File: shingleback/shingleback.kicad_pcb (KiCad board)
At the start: 2 copper layers, 117.8 x 86.2 mm, 45 parts

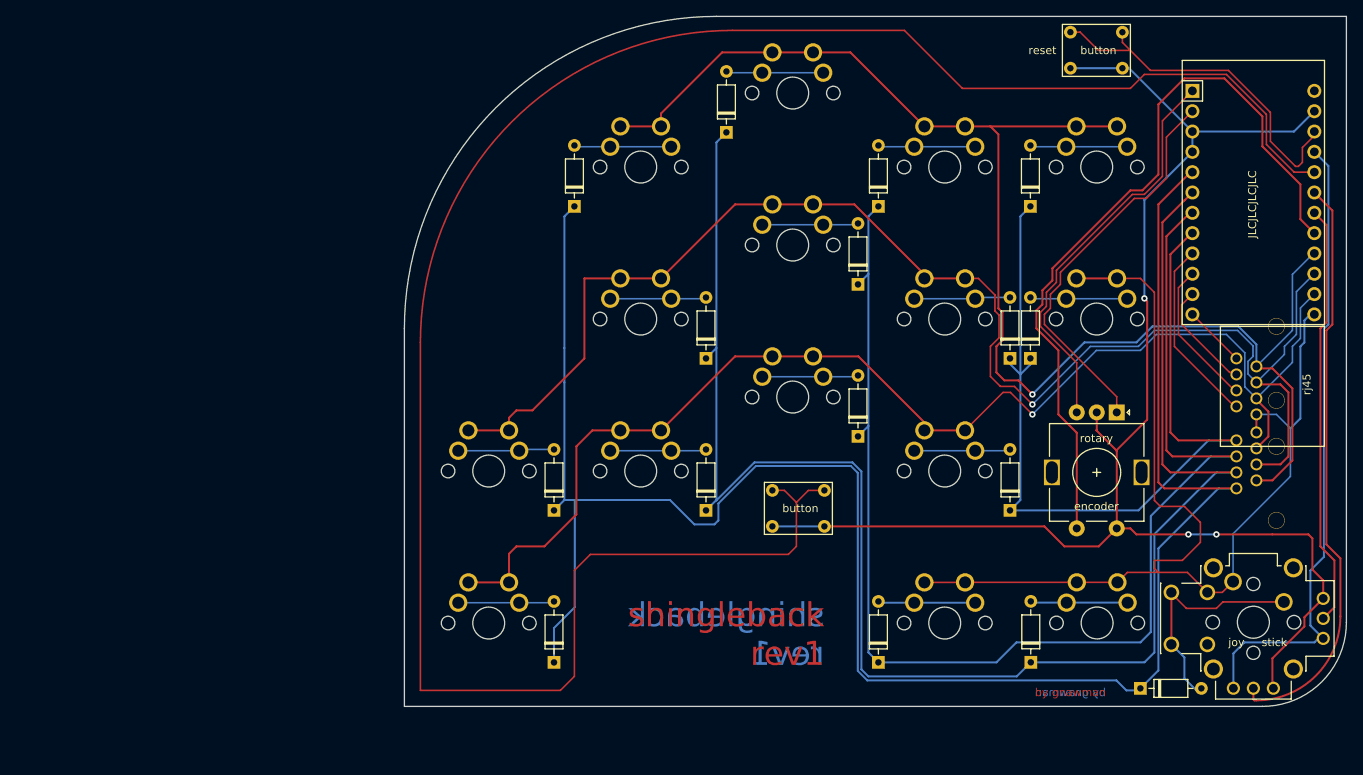
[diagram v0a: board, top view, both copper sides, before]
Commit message: shingleback rev2
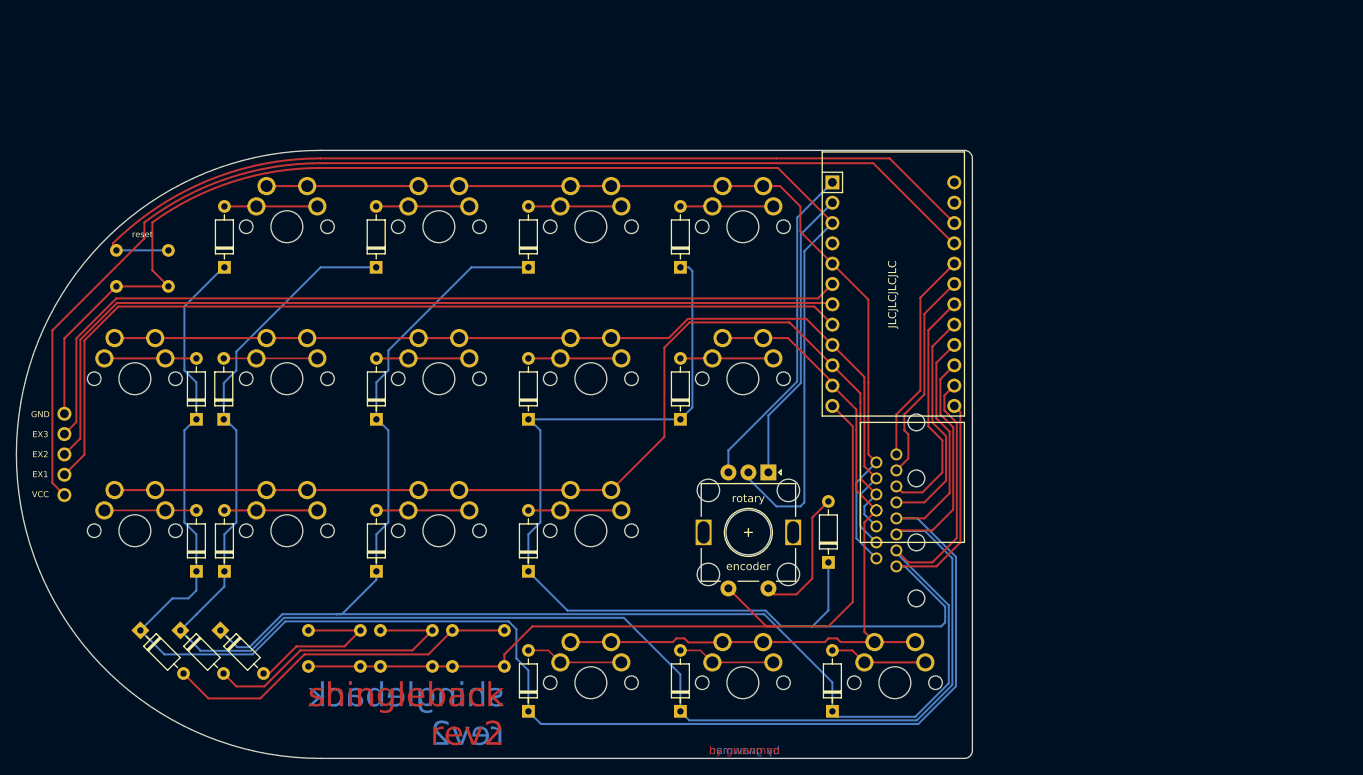
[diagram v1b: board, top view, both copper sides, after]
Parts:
- removed the ? at (125.0, 83.5)
- removed the ? at (162.2, 30.7)
- removed the ? at (118.5, 88.0)
- removed the ? at (125.0, 88.0)
- removed the ? at (155.8, 30.7)
- removed the ? at (118.5, 83.5)
- removed the ? at (155.8, 26.2)
- removed the ? at (162.2, 26.2)
- removed the R at (131.8, 105.0)
- removed the R at (150.8, 67.0)
- removed the R at (93.8, 48.0)
- removed the R at (164.5, 108.2)
- removed the R at (150.8, 105.0)
- removed the R at (129.2, 57.8)
- removed the R at (131.8, 48.0)
- removed the R at (148.2, 67.0)
- removed the R at (150.8, 48.0)
- removed the R at (110.2, 67.0)
- removed the R at (129.2, 76.8)
- removed the R at (91.2, 86.0)
- removed the R at (91.2, 105.0)
- removed the R at (112.8, 38.8)
- removed the R at (110.2, 86.0)
- removed the R at (148.2, 86.0)
- removed the REF at (185.0, 62.0)
- removed the REF at (185.0, 88.2)
- removed the REF** at (161.5, 73.8)
- removed the REF** at (183.7, 100.8)
- removed the REF** at (176.1, 94.9)
- removed the S14 at (159.0, 62.1)
- removed the S14 at (140.0, 62.1)
- removed the S14 at (121.0, 71.8)
- removed the S14 at (140.0, 81.1)
- removed the S14 at (102.0, 81.1)
- removed the S14 at (121.0, 52.8)
- removed the S14 at (140.0, 100.1)
- removed the S14 at (121.0, 33.8)
- removed the S14 at (102.0, 43.1)
- removed the S14 at (140.0, 43.1)
- removed the S14 at (159.1, 100.1)
- removed the S14 at (83.0, 81.1)
- removed the S14 at (102.0, 62.1)
- removed the S14 at (159.0, 43.1)
- removed the S14 at (83.0, 100.1)
- added ?: , , F.Cu at (76.0, 101.0)
- added ?: , , F.Cu at (76.0, 105.5)
- added ?: , , F.Cu at (36.5, 58.0)
- added ?: , , F.Cu at (43.0, 58.0)
- added ?: , , F.Cu at (60.5, 105.5)
- added ?: , , F.Cu at (30.0, 73.9)
- added ?: , , F.Cu at (30.0, 79.0)
- added ?: , , F.Cu at (30.0, 76.5)
- added ?: , , F.Cu at (69.5, 105.5)
- added ?: , , F.Cu at (36.5, 53.5)
- added ?: , , F.Cu at (43.0, 53.5)
- added ?: , , F.Cu at (67.0, 101.0)
- added ?: , , F.Cu at (60.5, 101.0)
- added ?: , , F.Cu at (30.0, 81.5)
- added ?: , , F.Cu at (78.5, 105.5)
- added ?: , , F.Cu at (69.5, 101.0)
- added ?: , , F.Cu at (85.0, 105.5)
- added ?: , , F.Cu at (30.0, 84.1)
- added ?: , , F.Cu at (78.5, 101.0)
- added ?: , , F.Cu at (67.0, 105.5)
- added ?: , , F.Cu at (85.0, 101.0)
- added R: d, Diode_THT:D_DO-35_SOD27_P7.62mm_Horizontal, F.Cu at (46.5, 93.6)
- added R: d, Diode_THT:D_DO-35_SOD27_P7.62mm_Horizontal, F.Cu at (46.5, 74.6)
- added R: d, Diode_THT:D_DO-35_SOD27_P7.62mm_Horizontal, F.Cu at (107.0, 111.1)
- added R: d, Diode_THT:D_DO-35_SOD27_P7.62mm_Horizontal, F.Cu at (39.5, 101.0)
- added R: d, Diode_THT:D_DO-35_SOD27_P7.62mm_Horizontal, F.Cu at (50.0, 55.6)
- added R: d, Diode_THT:D_DO-35_SOD27_P7.62mm_Horizontal, F.Cu at (69.0, 74.6)
- added R: d, Diode_THT:D_DO-35_SOD27_P7.62mm_Horizontal, F.Cu at (88.0, 111.1)
- added R: d, Diode_THT:D_DO-35_SOD27_P7.62mm_Horizontal, F.Cu at (50.0, 93.6)
- added R: d, Diode_THT:D_DO-35_SOD27_P7.62mm_Horizontal, F.Cu at (69.0, 55.6)
- added R: d, Diode_THT:D_DO-35_SOD27_P7.62mm_Horizontal, F.Cu at (107.0, 55.6)
- added R: d, Diode_THT:D_DO-35_SOD27_P7.62mm_Horizontal, F.Cu at (49.5, 101.0)
- added R: d, Diode_THT:D_DO-35_SOD27_P7.62mm_Horizontal, F.Cu at (125.5, 92.5)
- added R: d, Diode_THT:D_DO-35_SOD27_P7.62mm_Horizontal, F.Cu at (88.0, 74.6)
- added R: d, Diode_THT:D_DO-35_SOD27_P7.62mm_Horizontal, F.Cu at (49.9, 74.6)
- added R: d, Diode_THT:D_DO-35_SOD27_P7.62mm_Horizontal, F.Cu at (69.0, 93.6)
- added R: d, Diode_THT:D_DO-35_SOD27_P7.62mm_Horizontal, F.Cu at (126.0, 111.1)
- added R: d, Diode_THT:D_DO-35_SOD27_P7.62mm_Horizontal, F.Cu at (88.0, 93.6)
- added R: d, Diode_THT:D_DO-35_SOD27_P7.62mm_Horizontal, F.Cu at (44.5, 101.0)
- added R: d, Diode_THT:D_DO-35_SOD27_P7.62mm_Horizontal, F.Cu at (107.0, 74.6)
- added R: d, Diode_THT:D_DO-35_SOD27_P7.62mm_Horizontal, F.Cu at (88.0, 55.6)
- added REF: RJ45_gnawman, Connector_RJ:RJ45_gnawman, F.Cu at (140.0, 74.0)
- added REF: RJ45_gnawman, Connector_RJ:RJ45_gnawman, B.Cu at (140.0, 98.0)
- added REF**: RotaryEncoder_gnawman, Rotary_Encoder:RotaryEncoder_gnawman, F.Cu at (118.0, 81.2)
- added S14: , MX, F.Cu at (95.8, 107.5)
- added S14: , MX, F.Cu at (114.8, 50.5)
- added S14: , MX, F.Cu at (95.8, 69.5)
- added S14: , MX, F.Cu at (114.8, 107.5)
- added S14: , MX, F.Cu at (38.8, 88.5)
- added S14: , MX, F.Cu at (76.8, 88.5)
- added S14: , MX, F.Cu at (95.8, 50.5)
- added S14: , MX, F.Cu at (57.8, 88.5)
- added S14: , MX, F.Cu at (95.8, 88.5)
- added S14: , MX, F.Cu at (114.8, 69.5)
- added S14: , MX, F.Cu at (76.8, 50.5)
- added S14: , MX, F.Cu at (133.8, 107.5)
- added S14: , MX, F.Cu at (76.8, 69.5)
- added S14: , MX, F.Cu at (57.8, 50.5)
- added S14: , MX, F.Cu at (38.8, 69.5)
- added S14: , MX, F.Cu at (57.8, 69.5)
- moved MCU1 46.4 mm to (133.6, 59.0)
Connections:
- MCU1 pad 1: (no net) -> rot1
- MCU1 pad 10: col6 -> row3
- MCU1 pad 11: col7 -> row4
- MCU1 pad 12: col8 -> row5
- MCU1 pad 13: (no net) -> RAW
- MCU1 pad 14: GND -> (no net)
- MCU1 pad 15: (no net) -> RST
- MCU1 pad 17: (no net) -> col8
- MCU1 pad 18: (no net) -> col7
- MCU1 pad 19: (no net) -> col6
- MCU1 pad 2: (no net) -> rot2
- MCU1 pad 20: (no net) -> col5
- MCU1 pad 21: row1 -> col4
- MCU1 pad 22: row2 -> col3
- MCU1 pad 23: row3 -> col2
- MCU1 pad 24: row4 -> col1
- MCU1 pad 4: GND -> (no net)
- MCU1 pad 5: col1 -> row1
- MCU1 pad 6: col2 -> exp3
- MCU1 pad 7: col3 -> exp2
- MCU1 pad 8: col4 -> exp1
- MCU1 pad 9: col5 -> row2
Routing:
- net (no net): track 841.0 -> 306.1 mm
- net RST: track 0.00 -> 118.7 mm
- net exp1: track 0.00 -> 114.0 mm
- net col4: track 110.7 -> 224.5 mm
- net exp2: track 0.00 -> 110.9 mm
- net exp3: track 0.00 -> 109.9 mm
- net row5: track 0.00 -> 105.8 mm
- net col1: track 246.3 -> 160.9 mm
- net VCC: track 79.5 -> 146.3 mm
- net row1: track 180.5 -> 117.8 mm, vias 1 -> 0
- net row2: track 177.7 -> 120.7 mm, vias 1 -> 0
- net col3: track 165.6 -> 222.4 mm
- net row4: track 139.9 -> 95.8 mm
- net rot1: track 0.00 -> 41.6 mm
- net rot2: track 0.00 -> 37.0 mm
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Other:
- board size 117.8 x 86.2 mm -> 119.5 x 76 mm
- board text added: "EX1"
- board text added: "EX2"
- board text added: "EX3"
- board text added: "GND"
- board text added: "VCC"
- board text added: "shingleback rev2"
- board text removed: "button"
- board text removed: "empty"
- board text removed: "joy"
- board text removed: "rj45"
- board text removed: "shingleback rev1"
- board text removed: "stick"
- board text removed: "switch"
- board text removed: "this space intentionally left blank"
